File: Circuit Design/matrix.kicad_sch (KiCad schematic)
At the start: 198 parts

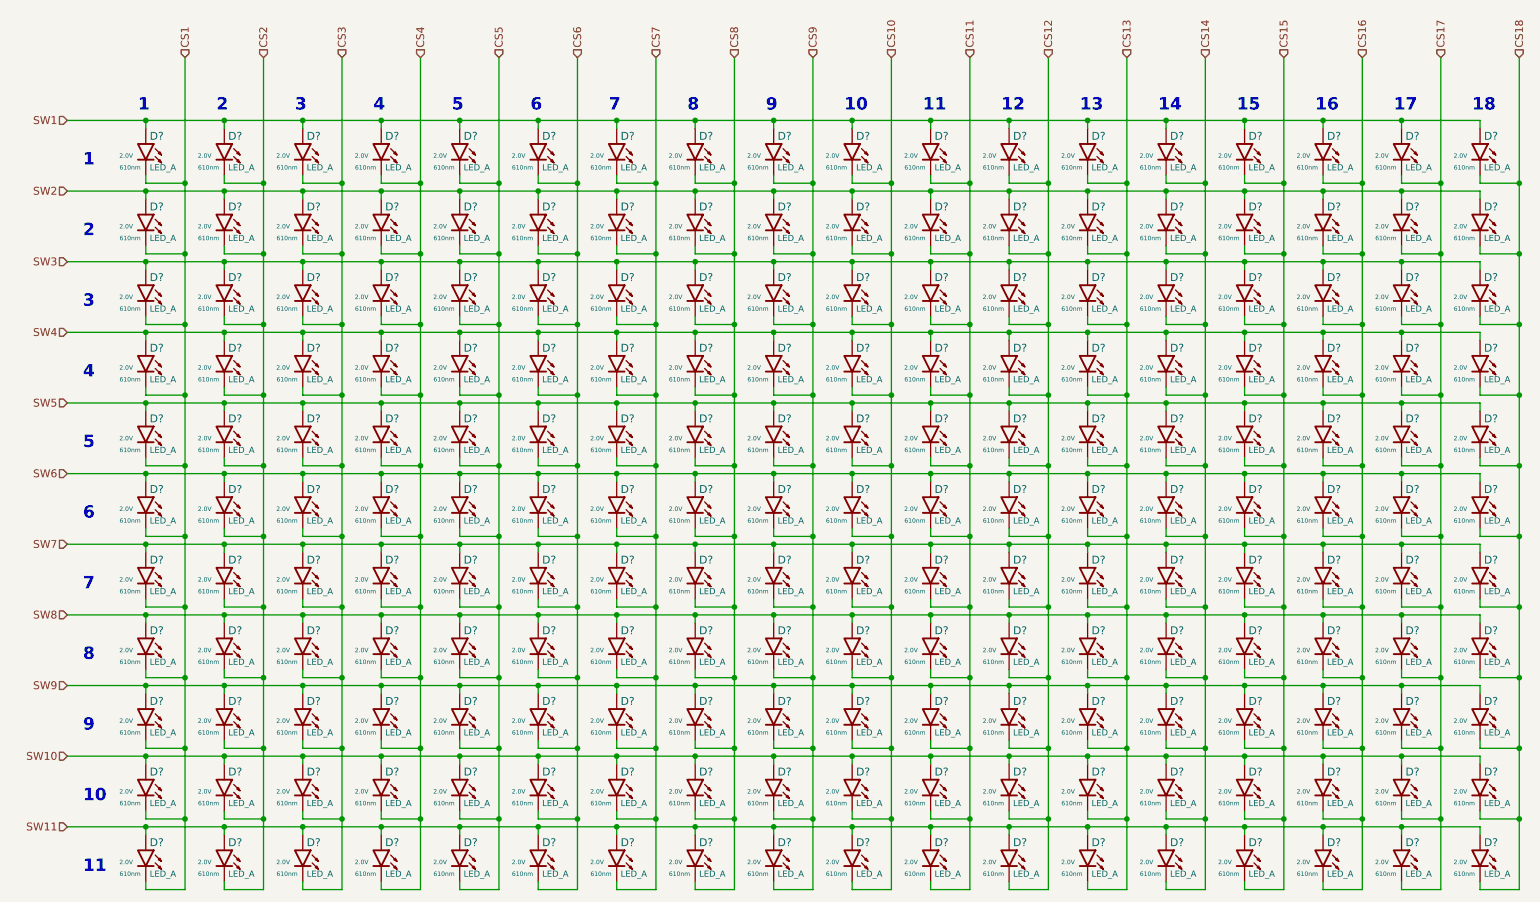
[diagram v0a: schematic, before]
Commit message: last commit before 0805 migration
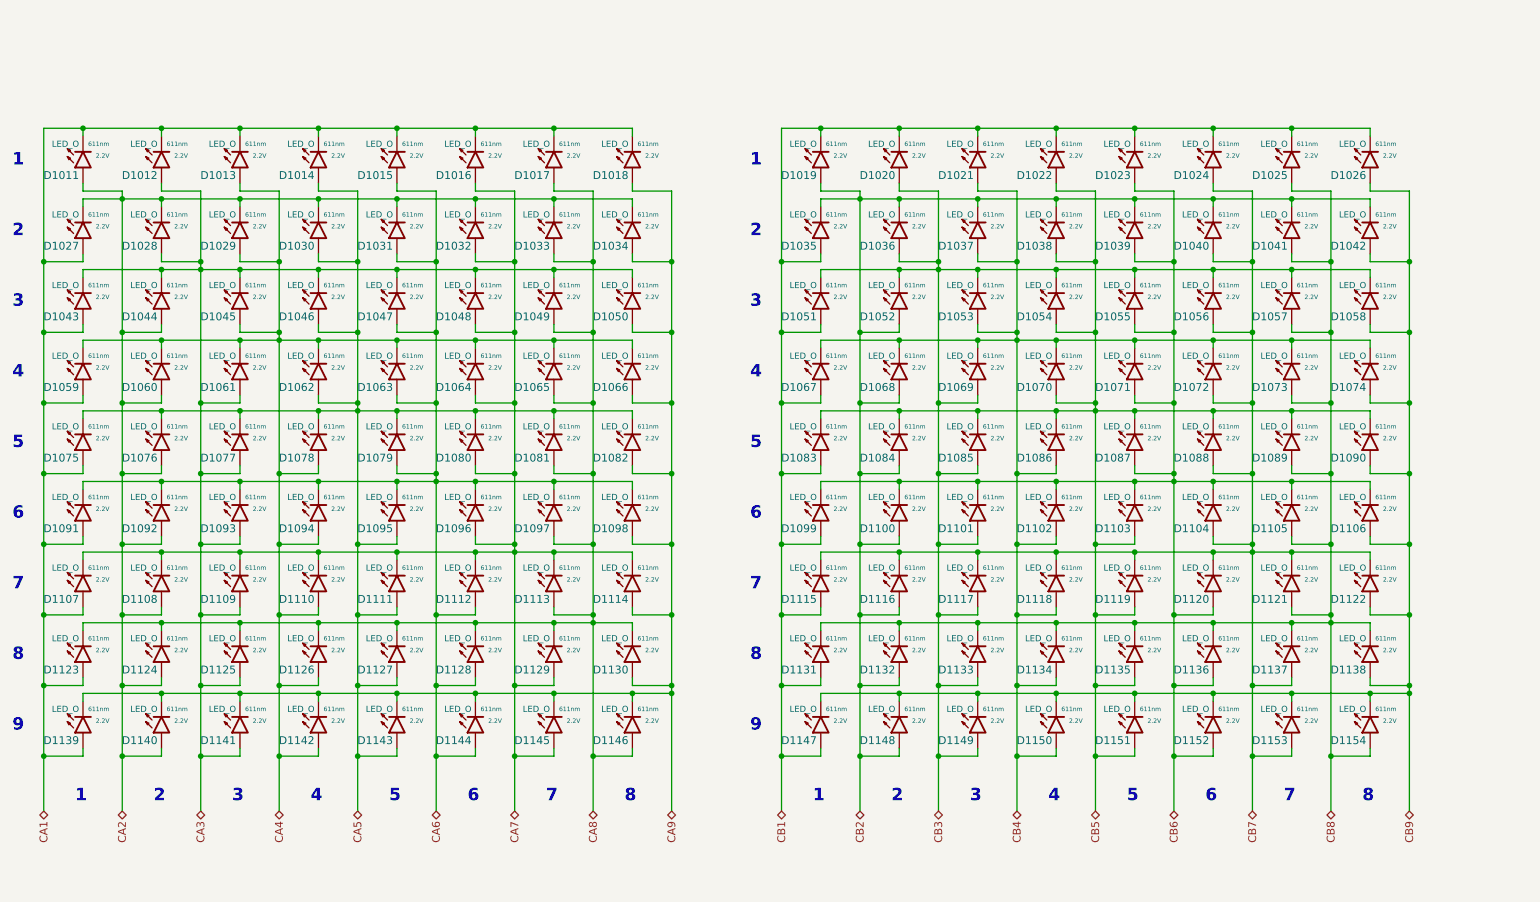
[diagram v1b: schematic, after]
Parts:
- removed D? (x198): LED_A, CoF_Diode:LED-0603, symbol CoE_Diode:LED_A
- added D1011, D1012, D1013, D1014, D1015, D1016, D1017, D1018, D1019, D1020, D1021, D1022, D1023, D1024, D1025, D1026, D1027, D1028, D1029, D1030, D1031, D1032, D1033, D1034, D1035, D1036, D1037, D1038, D1039, D1040, D1041, D1042, D1043, D1044, D1045, D1046, D1047, D1048, D1049, D1050, D1051, D1052, D1053, D1054, D1055, D1056, D1057, D1058, D1059, D1060, D1061, D1062, D1063, D1064, D1065, D1066, D1067, D1068, D1069, D1070, D1071, D1072, D1073, D1074, D1075, D1076, D1077, D1078, D1079, D1080, D1081, D1082, D1083, D1084, D1085, D1086, D1087, D1088, D1089, D1090, D1091, D1092, D1093, D1094, D1095, D1096, D1097, D1098, D1099, D1100, D1101, D1102, D1103, D1104, D1105, D1106, D1107, D1108, D1109, D1110, D1111, D1112, D1113, D1114, D1115, D1116, D1117, D1118, D1119, D1120, D1121, D1122, D1123, D1124, D1125, D1126, D1127, D1128, D1129, D1130, D1131, D1132, D1133, D1134, D1135, D1136, D1137, D1138, D1139, D1140, D1141, D1142, D1143, D1144, D1145, D1146, D1147, D1148, D1149, D1150, D1151, D1152, D1153, D1154: LED_O, CoF_Diode:LED-0402, symbol CoE_Diode:LED_O
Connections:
- new net CA1: D1011.1 (K), D1012.1 (K), D1013.1 (K), D1014.1 (K), D1015.1 (K), D1016.1 (K), D1017.1 (K), D1018.1 (K), D1027.2 (A), D1043.2 (A), D1059.2 (A), D1075.2 (A), D1091.2 (A), D1107.2 (A), D1123.2 (A), D1139.2 (A)
- new net CA2: D1011.2 (A), D1027.1 (K), D1028.1 (K), D1029.1 (K), D1030.1 (K), D1031.1 (K), D1032.1 (K), D1033.1 (K), D1034.1 (K), D1044.2 (A), D1060.2 (A), D1076.2 (A), D1092.2 (A), D1108.2 (A), D1124.2 (A), D1140.2 (A)
- new net CA3: D1012.2 (A), D1028.2 (A), D1043.1 (K), D1044.1 (K), D1045.1 (K), D1046.1 (K), D1047.1 (K), D1048.1 (K), D1049.1 (K), D1050.1 (K), D1061.2 (A), D1077.2 (A), D1093.2 (A), D1109.2 (A), D1125.2 (A), D1141.2 (A)
- new net CA4: D1013.2 (A), D1029.2 (A), D1045.2 (A), D1059.1 (K), D1060.1 (K), D1061.1 (K), D1062.1 (K), D1063.1 (K), D1064.1 (K), D1065.1 (K), D1066.1 (K), D1078.2 (A), D1094.2 (A), D1110.2 (A), D1126.2 (A), D1142.2 (A)
- new net CA5: D1014.2 (A), D1030.2 (A), D1046.2 (A), D1062.2 (A), D1075.1 (K), D1076.1 (K), D1077.1 (K), D1078.1 (K), D1079.1 (K), D1080.1 (K), D1081.1 (K), D1082.1 (K), D1095.2 (A), D1111.2 (A), D1127.2 (A), D1143.2 (A)
- new net CA6: D1015.2 (A), D1031.2 (A), D1047.2 (A), D1063.2 (A), D1079.2 (A), D1091.1 (K), D1092.1 (K), D1093.1 (K), D1094.1 (K), D1095.1 (K), D1096.1 (K), D1097.1 (K), D1098.1 (K), D1112.2 (A), D1128.2 (A), D1144.2 (A)
- new net CA7: D1016.2 (A), D1032.2 (A), D1048.2 (A), D1064.2 (A), D1080.2 (A), D1096.2 (A), D1107.1 (K), D1108.1 (K), D1109.1 (K), D1110.1 (K), D1111.1 (K), D1112.1 (K), D1113.1 (K), D1114.1 (K), D1129.2 (A), D1145.2 (A)
- new net CA8: D1017.2 (A), D1033.2 (A), D1049.2 (A), D1065.2 (A), D1081.2 (A), D1097.2 (A), D1113.2 (A), D1123.1 (K), D1124.1 (K), D1125.1 (K), D1126.1 (K), D1127.1 (K), D1128.1 (K), D1129.1 (K), D1130.1 (K), D1146.2 (A)
- new net CA9: D1018.2 (A), D1034.2 (A), D1050.2 (A), D1066.2 (A), D1082.2 (A), D1098.2 (A), D1114.2 (A), D1130.2 (A), D1139.1 (K), D1140.1 (K), D1141.1 (K), D1142.1 (K), D1143.1 (K), D1144.1 (K), D1145.1 (K), D1146.1 (K)
- new net CB1: D1019.1 (K), D1020.1 (K), D1021.1 (K), D1022.1 (K), D1023.1 (K), D1024.1 (K), D1025.1 (K), D1026.1 (K), D1035.2 (A), D1051.2 (A), D1067.2 (A), D1083.2 (A), D1099.2 (A), D1115.2 (A), D1131.2 (A), D1147.2 (A)
- new net CB2: D1019.2 (A), D1035.1 (K), D1036.1 (K), D1037.1 (K), D1038.1 (K), D1039.1 (K), D1040.1 (K), D1041.1 (K), D1042.1 (K), D1052.2 (A), D1068.2 (A), D1084.2 (A), D1100.2 (A), D1116.2 (A), D1132.2 (A), D1148.2 (A)
- new net CB3: D1020.2 (A), D1036.2 (A), D1051.1 (K), D1052.1 (K), D1053.1 (K), D1054.1 (K), D1055.1 (K), D1056.1 (K), D1057.1 (K), D1058.1 (K), D1069.2 (A), D1085.2 (A), D1101.2 (A), D1117.2 (A), D1133.2 (A), D1149.2 (A)
- new net CB4: D1021.2 (A), D1037.2 (A), D1053.2 (A), D1067.1 (K), D1068.1 (K), D1069.1 (K), D1070.1 (K), D1071.1 (K), D1072.1 (K), D1073.1 (K), D1074.1 (K), D1086.2 (A), D1102.2 (A), D1118.2 (A), D1134.2 (A), D1150.2 (A)
- new net CB5: D1022.2 (A), D1038.2 (A), D1054.2 (A), D1070.2 (A), D1083.1 (K), D1084.1 (K), D1085.1 (K), D1086.1 (K), D1087.1 (K), D1088.1 (K), D1089.1 (K), D1090.1 (K), D1103.2 (A), D1119.2 (A), D1135.2 (A), D1151.2 (A)
- new net CB6: D1023.2 (A), D1039.2 (A), D1055.2 (A), D1071.2 (A), D1087.2 (A), D1099.1 (K), D1100.1 (K), D1101.1 (K), D1102.1 (K), D1103.1 (K), D1104.1 (K), D1105.1 (K), D1106.1 (K), D1120.2 (A), D1136.2 (A), D1152.2 (A)
- new net CB7: D1024.2 (A), D1040.2 (A), D1056.2 (A), D1072.2 (A), D1088.2 (A), D1104.2 (A), D1115.1 (K), D1116.1 (K), D1117.1 (K), D1118.1 (K), D1119.1 (K), D1120.1 (K), D1121.1 (K), D1122.1 (K), D1137.2 (A), D1153.2 (A)
- new net CB8: D1025.2 (A), D1041.2 (A), D1057.2 (A), D1073.2 (A), D1089.2 (A), D1105.2 (A), D1121.2 (A), D1131.1 (K), D1132.1 (K), D1133.1 (K), D1134.1 (K), D1135.1 (K), D1136.1 (K), D1137.1 (K), D1138.1 (K), D1154.2 (A)
- new net CB9: D1026.2 (A), D1042.2 (A), D1058.2 (A), D1074.2 (A), D1090.2 (A), D1106.2 (A), D1122.2 (A), D1138.2 (A), D1147.1 (K), D1148.1 (K), D1149.1 (K), D1150.1 (K), D1151.1 (K), D1152.1 (K), D1153.1 (K), D1154.1 (K)
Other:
- note removed: "10"
- note removed: "11"
- note removed: "12"
- note removed: "13"
- note removed: "14"
- note removed: "15"
- note removed: "16"
- note removed: "17"
- note removed: "18"
